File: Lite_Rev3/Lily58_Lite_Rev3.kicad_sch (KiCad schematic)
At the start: 118 parts, among them J1 M2HOLE, J10 LOGO, J10 M2HOLE, J11 LOGO, J11 M2HOLE, J12 HOLE, J13 HOLE, J14 HOLE, J15 HOLE, J16 OLED_R, J19 breakaway, J2 M2HOLE, J20 breakaway, J21 breakaway, J22 AudioJack4, J22 breakaway, J3 HOLE, J4 HOLE, J5 HOLE, J6 HOLE, J7 OLED_L, J9 AudioJack4, SW1 SW_Push, SW10 SW_Push, SW11 SW_Push, SW12 SW_Push, SW13 SW_Push, SW14 SW_Push, SW15 SW_Push, SW16 SW_Push, SW17 SW_Push, SW18 SW_Push, SW19 SW_Push, SW2 SW_Push, SW20 SW_Push, SW21 SW_Push, SW22 SW_Push, SW23 SW_Push, SW24 SW_Push, SW25 SW_Push, SW26 SW_Push, SW27 SW_Push, SW28 SW_Push, SW29 SW_Push, SW3 SW_Push, SW30 SW_Push, SW31 SW_Push, SW32 SW_Push, SW33 SW_Push, SW34 SW_Push, SW35 SW_Push, SW36 SW_Push, SW37 SW_Push, SW38 SW_Push, SW39 SW_Push, SW4 SW_Push, SW40 SW_Push, SW41 SW_Push, SW42 SW_Push, SW43 SW_Push, SW44 SW_Push, SW45 SW_Push, SW46 SW_Push, SW47 SW_Push, SW48 SW_Push, SW49 SW_Push, SW5 SW_Push, SW50 SW_Push, SW51 SW_Push, SW52 SW_Push, SW53 SW_Push, SW54 SW_Push, SW55 SW_Push, SW56 SW_Push, SW57 SW_Push, SW58 SW_Push, SW6 SW_Push, SW7 SW_Push, SW8 SW_Push, SW9 SW_Push

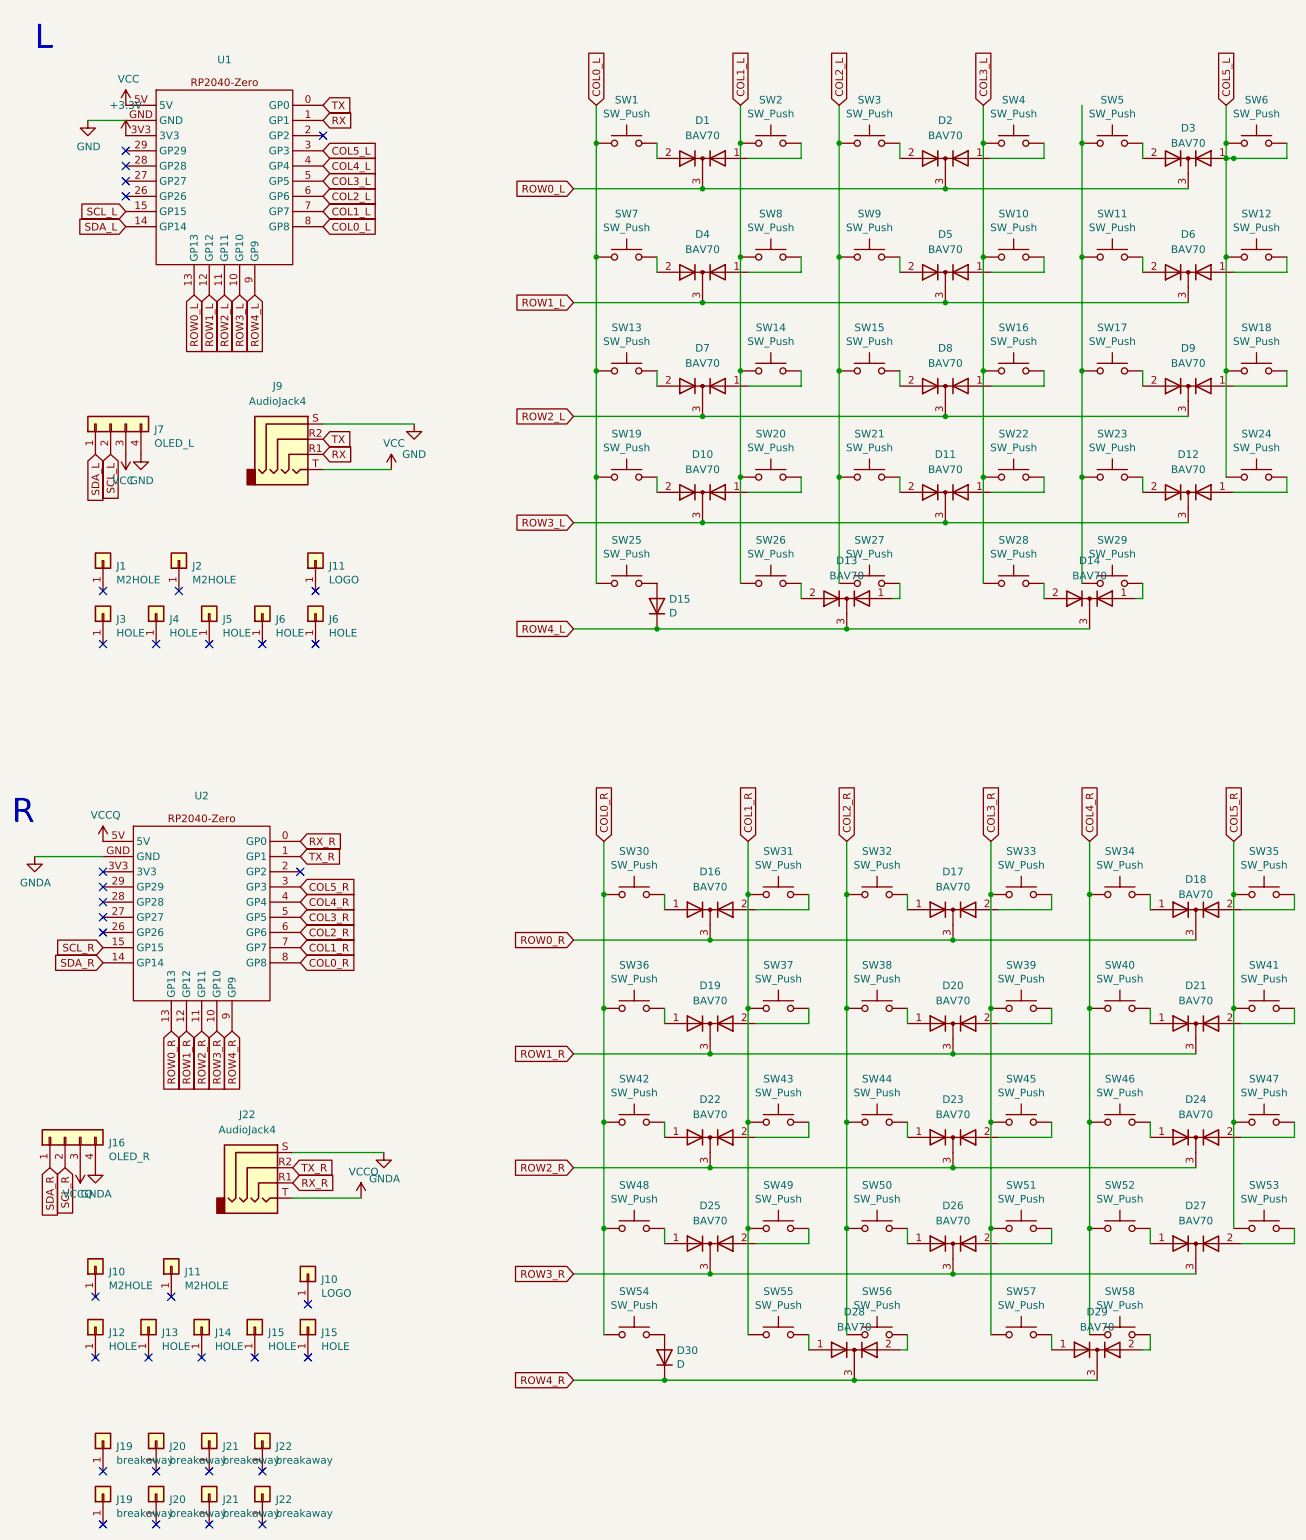
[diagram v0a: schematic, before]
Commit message: [Lily58 Lite Rev3] fix PCB
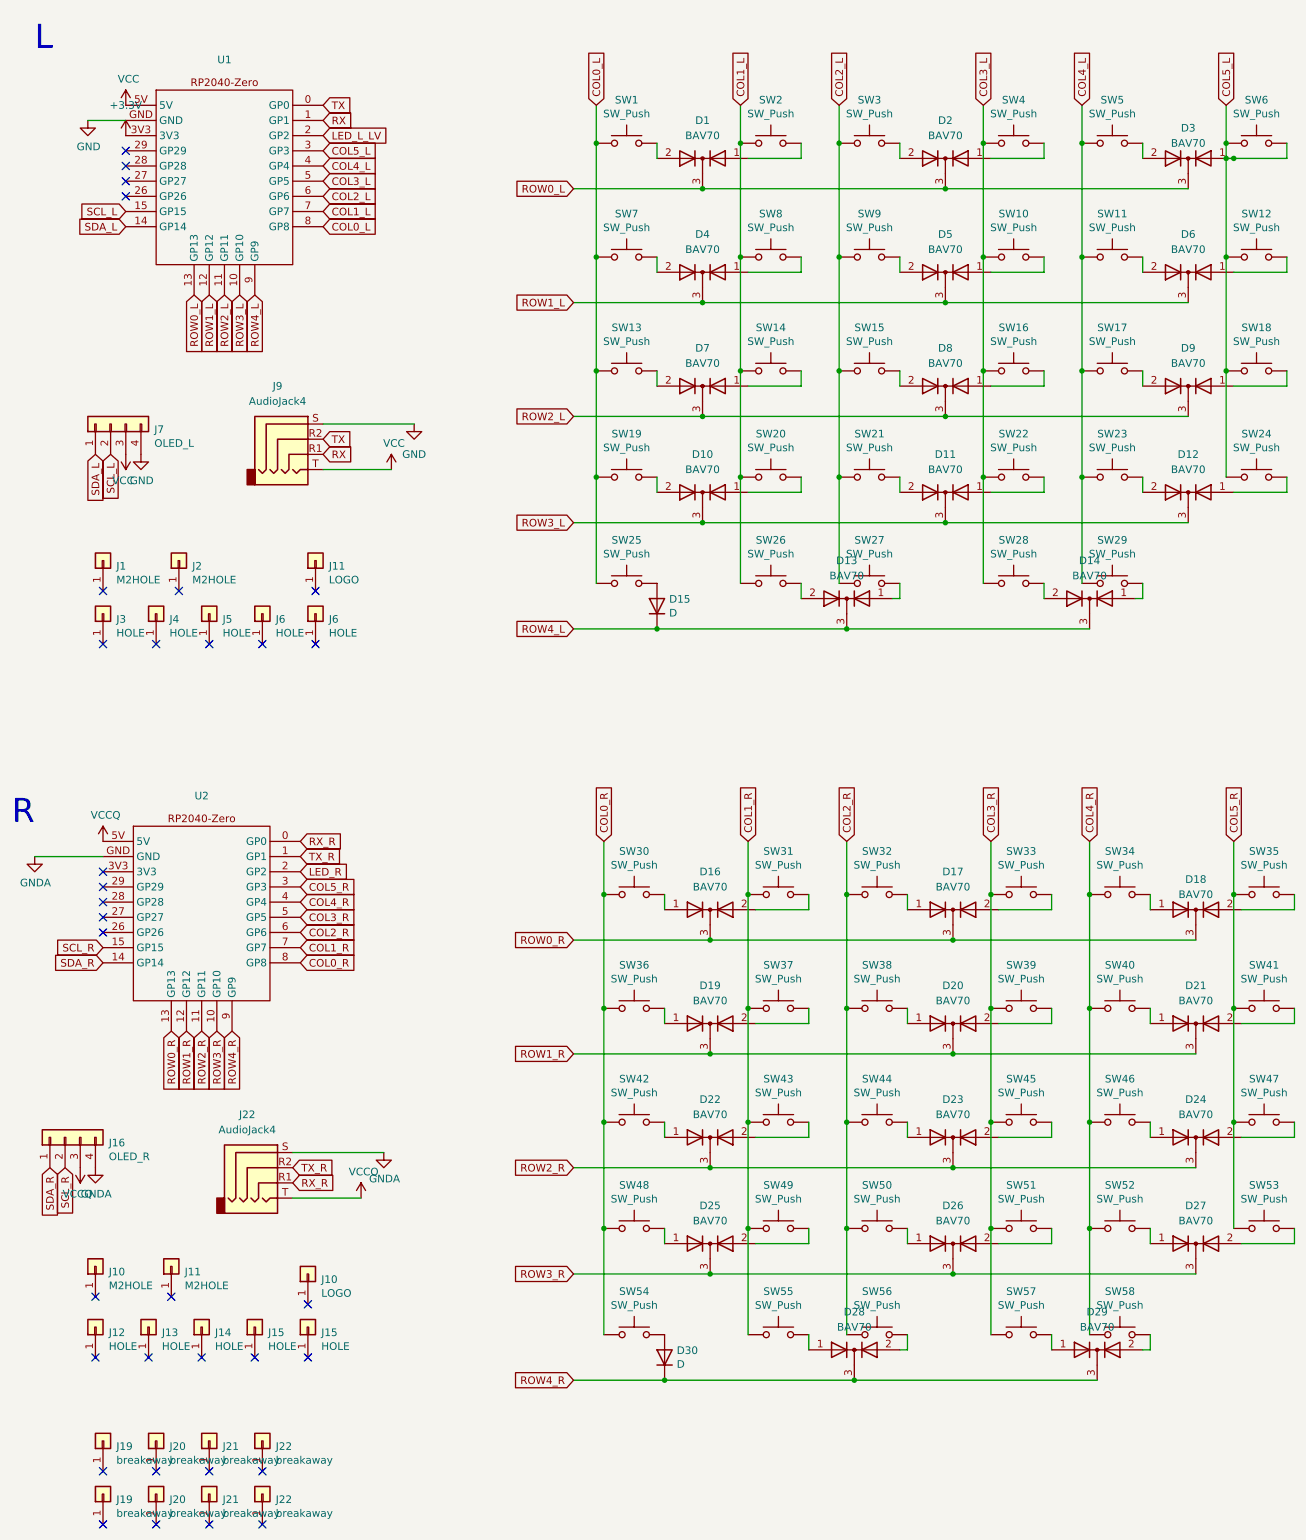
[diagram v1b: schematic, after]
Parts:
- J12, J13, J14, J15, J3, J4, J5, J6: footprint yuchi:HOLE_M2_TH_5mm -> yuchi:HOLE_M2_TH
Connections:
- net COL4_L: now also SW11.1, SW17.1, SW23.1, SW29.1, SW5.1
- net LED_L_LV: now reaches U1.2 (GP2)
- net LED_R: now reaches U2.2 (GP2)
- no-connect marks 35 -> 33
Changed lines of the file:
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@@
   (title_block
     (title "Lily58 Lite Rev3")
-    (date "2024-09-07")
+    (date "2024-07-18")
   )
   (junction (at 160.02 166.37) (diameter 0) (color 0 0 0 0)
@@
   (no_connect (at 76.2 262.89))
   (no_connect (at 93.98 124.46))
-  (no_connect (at 109.22 162.56))
   (no_connect (at 80.01 46.99))
   (no_connect (at 76.2 170.18))
@@
   (no_connect (at 92.71 243.84))
   (no_connect (at 101.6 243.84))
-  (no_connect (at 113.03 39.37))
   (no_connect (at 85.09 124.46))
   (no_connect (at 93.98 271.78))
@@
     )
   )
+  (global_label "LED_R" (shape input) (at 109.22 162.56 0)
+    (effects (font (size 1.27 1.27)) (justify left))
+    (property "Intersheetrefs" "${INTERSHEET_REFS}" (at 109.22 162.56 0)
+      (effects (font (size 1.27 1.27)) hide)
+    )
+  )
   (global_label "TX_R" (shape input) (at 109.22 160.02 0) (fields_autoplaced)
     (effects (font (size 1.27 1.27)) (justify left))
@@
     )
   )
+  (global_label "COL4_L" (shape input) (at 240.03 34.29 90) (fields_autoplaced)
+    (effects (font (size 1.27 1.27)) (justify left))
+    (property "Intersheetrefs" "${INTERSHEET_REFS}" (at 240.03 24.471 90)
+      (effects (font (size 1.27 1.27)) (justify left) hide)
+    )
+  )
+  (global_label "LED_L_LV" (shape input) (at 113.03 39.37 0)
+    (effects (font (size 1.27 1.27)) (justify left))
+    (property "Intersheetrefs" "${INTERSHEET_REFS}" (at 113.03 39.37 0)
+      (effects (font (size 1.27 1.27)) hide)
+    )
+  )
   (global_label "ROW4_R" (shape input) (at 97.79 189.23 270)
     (effects (font (size 1.27 1.27)) (justify right))
@@
       (effects (font (size 1.27 1.27)) (justify right))
     )
-    (property "Footprint" "yuchi:HOLE_M2_TH_5mm" (at 92.71 238.76 0)
+    (property "Footprint" "yuchi:HOLE_M2_TH" (at 92.71 238.76 0)
       (effects (font (size 1.27 1.27)) hide)
     )
@@
       (effects (font (size 1.27 1.27)) (justify right))
     )
-    (property "Footprint" "yuchi:HOLE_M2_TH_5mm" (at 102.87 119.38 0)
+    (property "Footprint" "yuchi:HOLE_M2_TH" (at 102.87 119.38 0)
       (effects (font (size 1.27 1.27)) hide)
     )
@@
       (effects (font (size 1.27 1.27)) (justify right))
     )
-    (property "Footprint" "yuchi:HOLE_M2_TH_5mm" (at 83.82 238.76 0)
+    (property "Footprint" "yuchi:HOLE_M2_TH" (at 83.82 238.76 0)
       (effects (font (size 1.27 1.27)) hide)
     )
@@
       (effects (font (size 1.27 1.27)) (justify right))
     )
-    (property "Footprint" "yuchi:HOLE_M2_TH_5mm" (at 76.2 119.38 0)
+    (property "Footprint" "yuchi:HOLE_M2_TH" (at 76.2 119.38 0)
       (effects (font (size 1.27 1.27)) hide)
     )
@@
       (effects (font (size 1.27 1.27)) (justify right))
     )
-    (property "Footprint" "yuchi:HOLE_M2_TH_5mm" (at 74.93 238.76 0)
+    (property "Footprint" "yuchi:HOLE_M2_TH" (at 74.93 238.76 0)
       (effects (font (size 1.27 1.27)) hide)
     )
@@
       (effects (font (size 1.27 1.27)) (justify right))
     )
-    (property "Footprint" "yuchi:HOLE_M2_TH_5mm" (at 93.98 119.38 0)
+    (property "Footprint" "yuchi:HOLE_M2_TH" (at 93.98 119.38 0)
       (effects (font (size 1.27 1.27)) hide)
     )
@@
       (effects (font (size 1.27 1.27)) (justify right))
     )
-    (property "Footprint" "yuchi:HOLE_M2_TH_5mm" (at 85.09 119.38 0)
+    (property "Footprint" "yuchi:HOLE_M2_TH" (at 85.09 119.38 0)
       (effects (font (size 1.27 1.27)) hide)
     )
@@
       (effects (font (size 1.27 1.27)) (justify right))
     )
-    (property "Footprint" "yuchi:HOLE_M2_TH_5mm" (at 101.6 238.76 0)
+    (property "Footprint" "yuchi:HOLE_M2_TH" (at 101.6 238.76 0)
       (effects (font (size 1.27 1.27)) hide)
     )
